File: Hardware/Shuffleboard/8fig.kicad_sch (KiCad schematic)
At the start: 22 parts, among them U4 INND-TS56RCB, U5 INND-TS56RCB, U6 LOGIC-74HC595N_DIP16_, U8 LOGIC-74HC595N_DIP16_

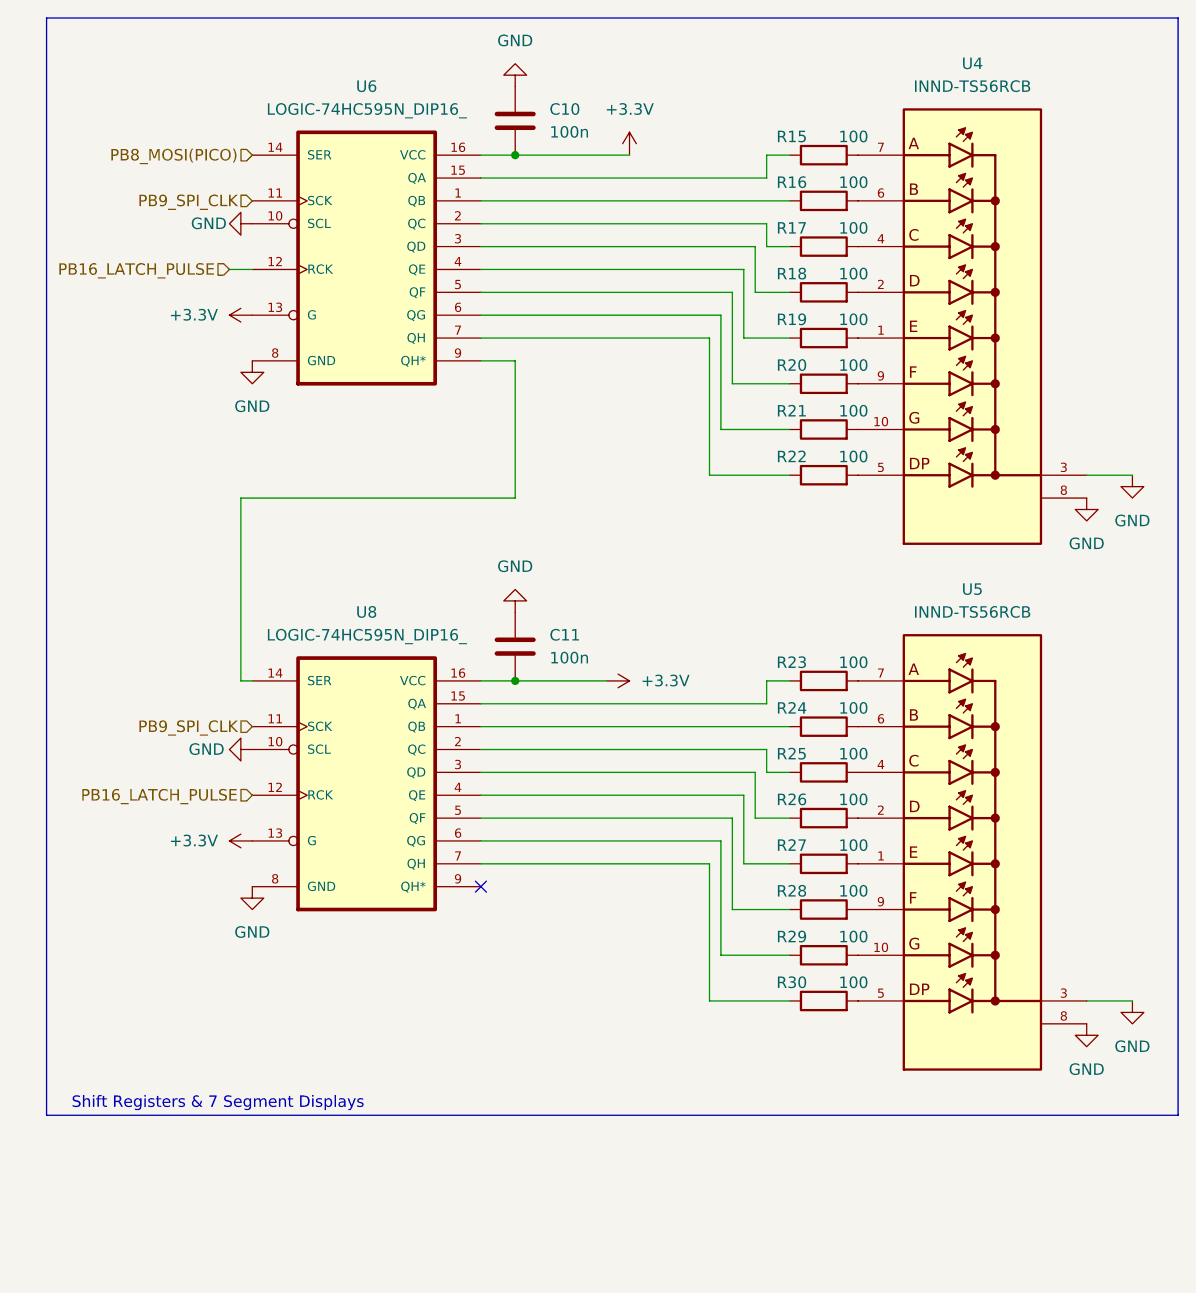
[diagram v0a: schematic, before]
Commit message: layout 2
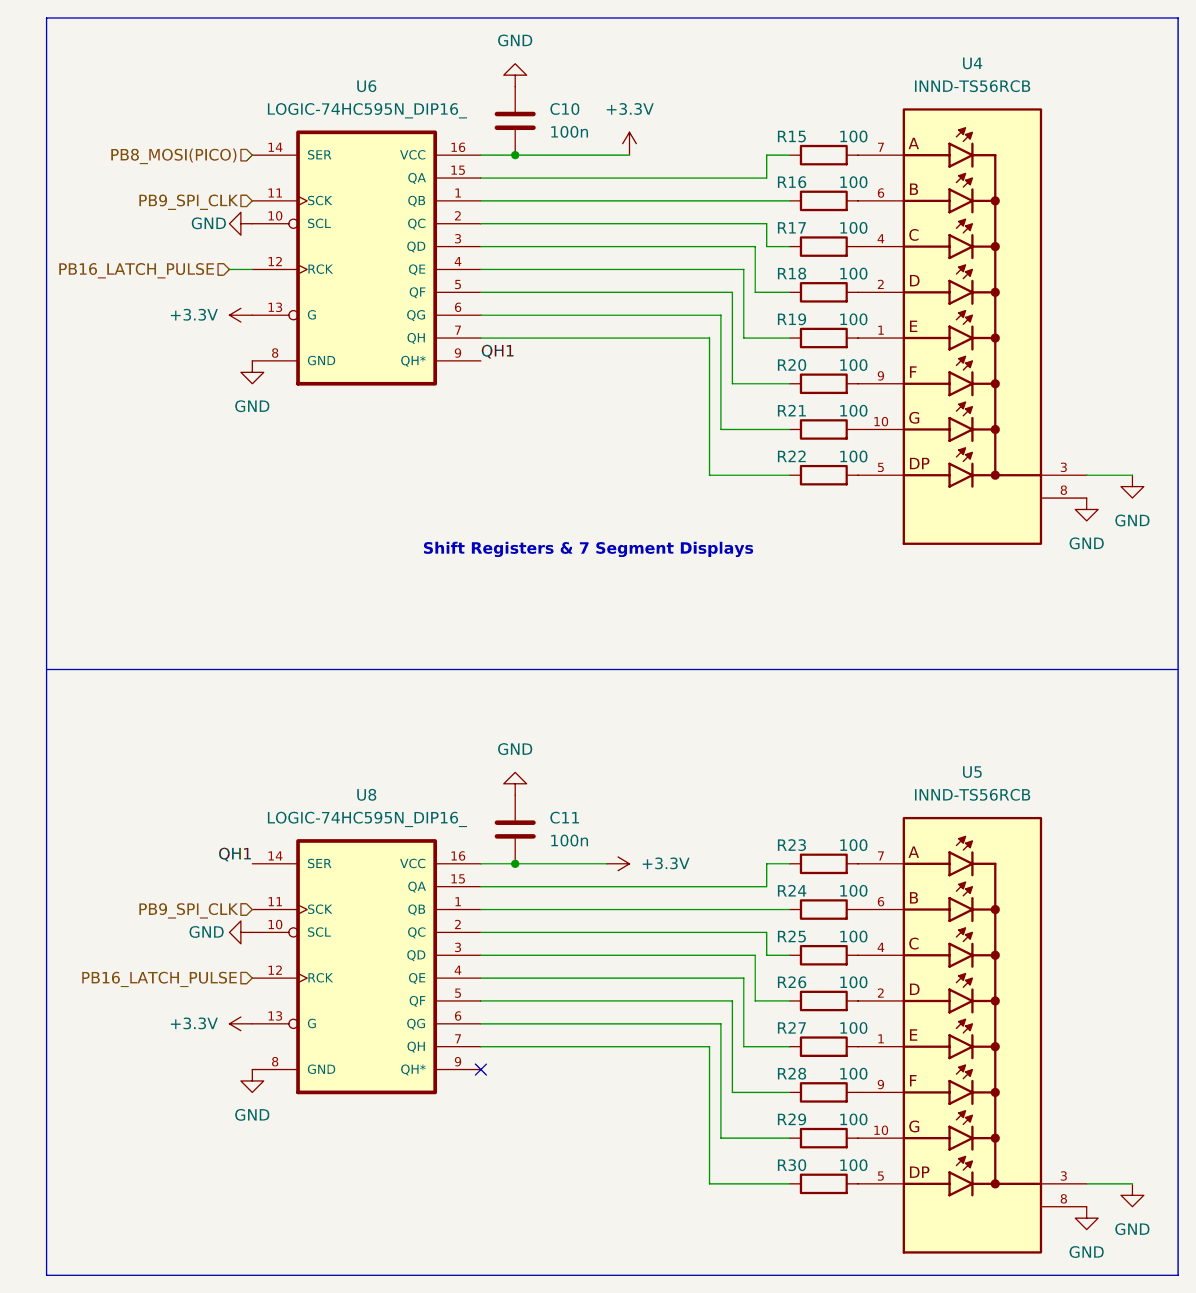
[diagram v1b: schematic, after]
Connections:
- net QH1: now reaches U6.9 (QH*), U8.14 (SER)
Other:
- moved on the sheet: C11, R23, R24, R25, R26, R27, R28, R29, R30, U5, U8
